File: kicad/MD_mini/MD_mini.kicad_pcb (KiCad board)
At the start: 2 copper layers, 58.6 x 36.3 mm, 49 parts, among them J1 Conn_01x02_Pin, J2 Conn_01x03_Pin, J3 Conn_01x02_Pin, J4 Conn_01x02_Pin, J6 Conn_02x03_Odd_Even, U1 IRS2003, U2 SCM3723ASA, U3 IRS2003, U4 ACS711xEXLT-15AB, U7 IRS2003, U8 IRS2003, U9 SCM3723ASA

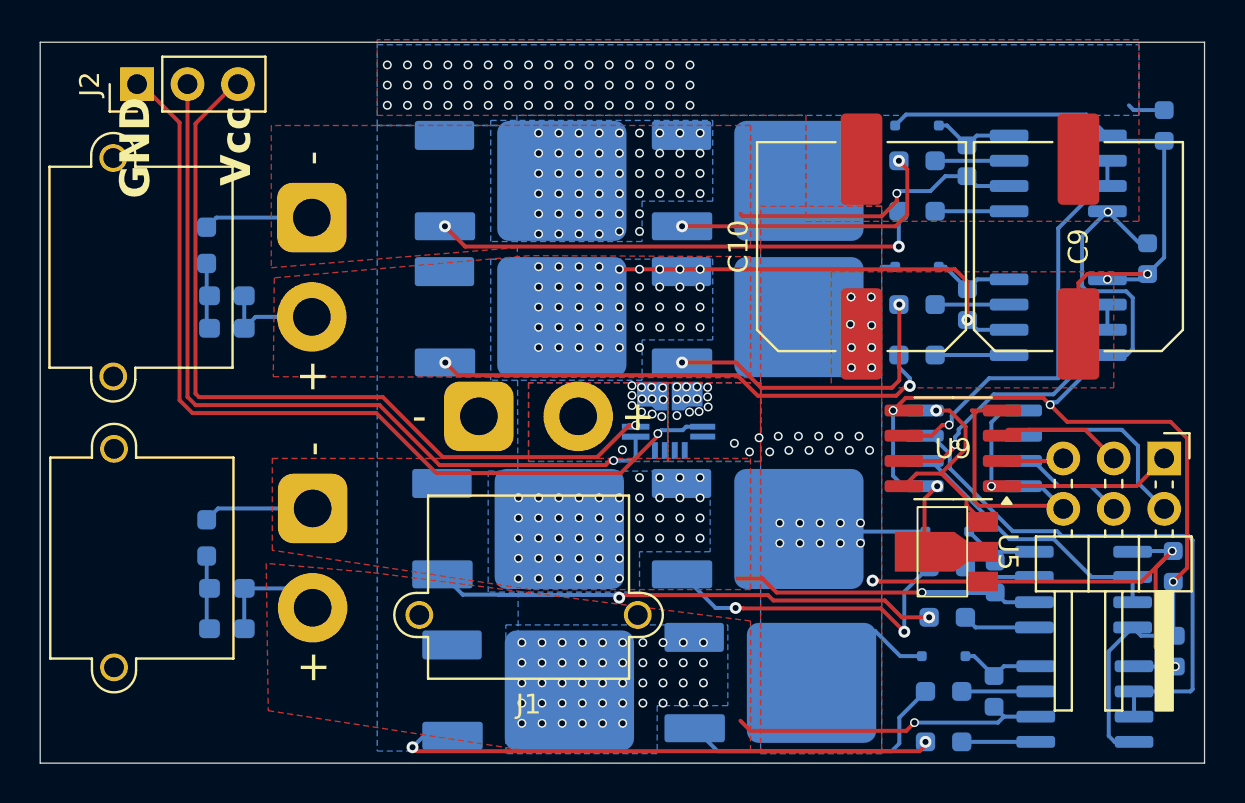
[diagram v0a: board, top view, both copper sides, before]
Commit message: a
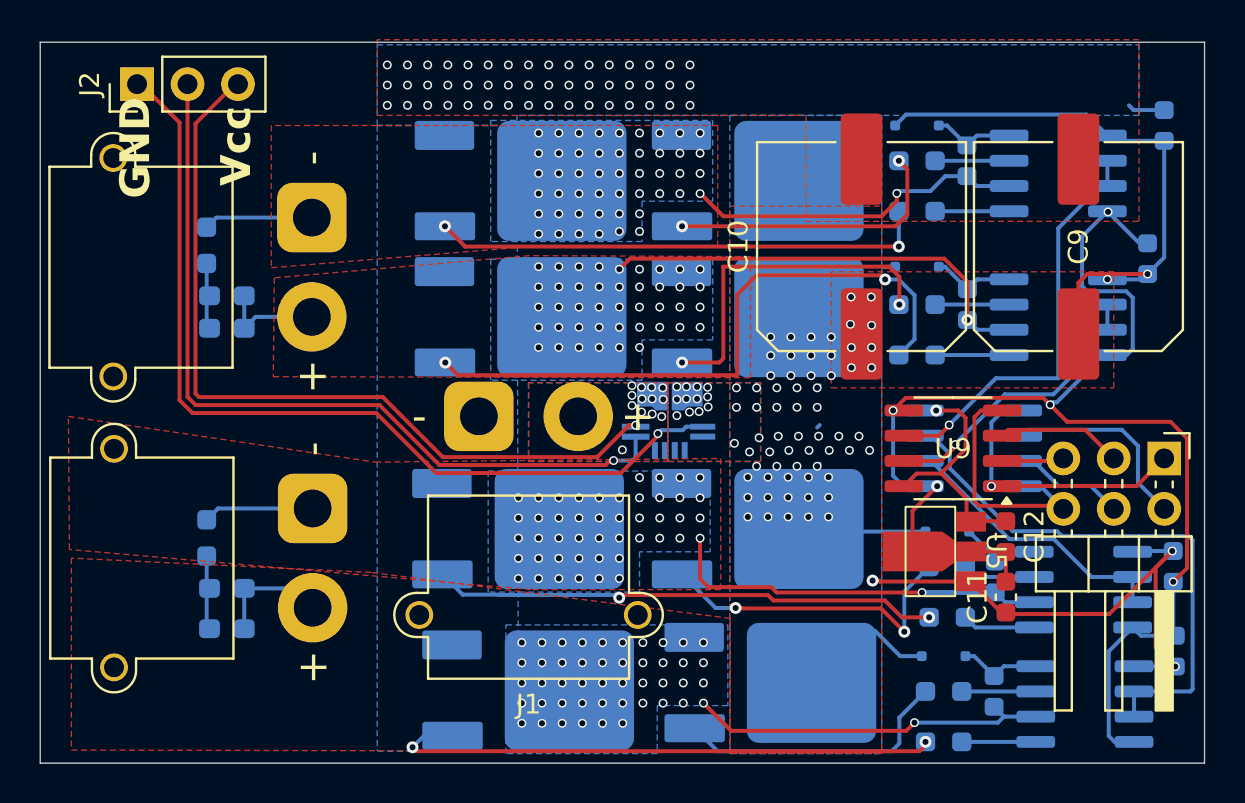
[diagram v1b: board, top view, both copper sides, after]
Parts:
- added C11: min0.33u, Capacitor_SMD:C_0603_1608Metric, F.Cu at (187.1, 122.3)
- added C12: 0.1u, Capacitor_SMD:C_0603_1608Metric, F.Cu at (187.1, 119.2)
- moved U5 0.60 mm to (186.1, 120.0)
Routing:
- net Net-(Q2-G): track 26.1 -> 32.1 mm
- net ch2_1: track 24.7 -> 28.6 mm
- net GND: track 64.4 -> 67.9 mm
- net ch1_1: track 20.3 -> 22.8 mm
- net VCC: track 63.9 -> 66.2 mm, vias 49 -> 80
- net ch2_2: track 22.0 -> 24.2 mm
- net Net-(Q1-G): track 15.4 -> 17.3 mm
- net Net-(U2-VCC2): track 10.8 -> 12.5 mm
